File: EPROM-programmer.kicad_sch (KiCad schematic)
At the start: 34 parts, among them J1 ZIF-socket, J2 ISP, J3 DAC_A, J4 DAC_B, J5 GND, P1 USB-C, SW1 SW_Push, U1 ATmega1284-P, U2 MCP2221AxP, U3 MCP4812, Y1 20M

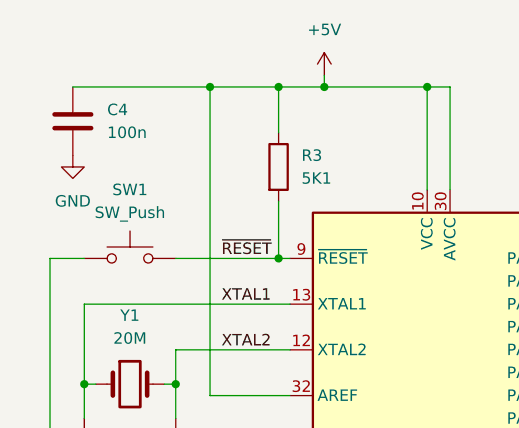
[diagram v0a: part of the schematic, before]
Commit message: Fix capacitor-stuff
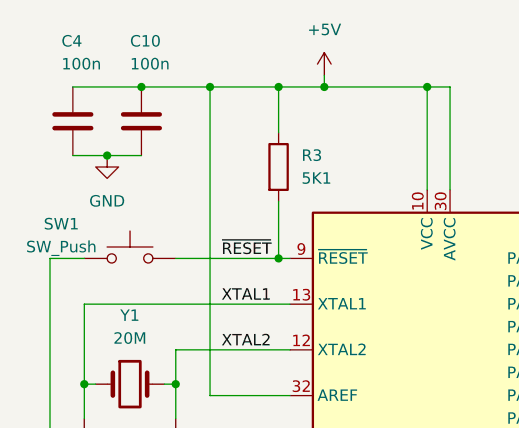
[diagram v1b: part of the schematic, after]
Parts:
- added C10: 100n, Capacitor_THT:C_Rect_L4.6mm_W3.0mm_P2.50mm_MKS02_FKP02, symbol Device:C
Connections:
- net +5V: now also C10.1
- net GND: now also C10.2
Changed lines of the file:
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@@
   (junction (at 99.06 157.48) (diameter 0) (color 0 0 0 0)
   )
+  (junction (at 25.4 35.56) (diameter 0) (color 0 0 0 0)
+  )
   (junction (at 180.34 154.94) (diameter 0) (color 0 0 0 0)
   )
@@
   )
   (junction (at 195.58 121.92) (diameter 0) (color 0 0 0 0)
+  )
+  (junction (at 21.59 43.18) (diameter 0) (color 0 0 0 0)
   )
   (junction (at 233.68 106.68) (diameter 0) (color 0 0 0 0)
@@
     (stroke (width 0) (type default))
   )
+  (wire (pts (xy 21.59 43.18) (xy 25.4 43.18))
+    (stroke (width 0) (type default))
+  )
   (wire (pts (xy 72.39 72.39) (xy 80.01 72.39))
     (stroke (width 0) (type default))
@@
     (stroke (width 0) (type default))
   )
-  (wire (pts (xy 17.78 35.56) (xy 33.02 35.56))
+  (wire (pts (xy 17.78 35.56) (xy 25.4 35.56))
     (stroke (width 0) (type default))
   )
@@
     (stroke (width 0) (type default))
   )
+  (wire (pts (xy 17.78 43.18) (xy 21.59 43.18))
+    (stroke (width 0) (type default))
+  )
   (wire (pts (xy 195.58 121.92) (xy 215.9 121.92))
     (stroke (width 0) (type default))
@@
     (stroke (width 0) (type default))
   )
+  (wire (pts (xy 25.4 35.56) (xy 33.02 35.56))
+    (stroke (width 0) (type default))
+  )
   (wire (pts (xy 132.08 176.53) (xy 143.51 176.53))
     (stroke (width 0) (type default))
@@
   )
   (symbol (lib_id "Device:C") (at 17.78 39.37 0) (unit 1)
-    (in_bom yes) (on_board yes) (dnp no) (fields_autoplaced)
-    (property "Reference" "C4" (at 21.59 38.1 0)
-      (effects (font (size 1.27 1.27)) (justify left))
-    )
-    (property "Value" "100n" (at 21.59 40.64 0)
+    (in_bom yes) (on_board yes) (dnp no)
+    (property "Reference" "C4" (at 16.51 30.48 0)
+      (effects (font (size 1.27 1.27)) (justify left))
+    )
+    (property "Value" "100n" (at 16.51 33.02 0)
       (effects (font (size 1.27 1.27)) (justify left))
     )
@@
     )
   )
-  (symbol (lib_id "power:GND") (at 17.78 43.18 0) (unit 1)
-    (in_bom yes) (on_board yes) (dnp no) (fields_autoplaced)
-    (property "Reference" "#PWR015" (at 17.78 49.53 0)
-      (effects (font (size 1.27 1.27)) hide)
-    )
-    (property "Value" "GND" (at 17.78 48.26 0)
-      (effects (font (size 1.27 1.27)))
-    )
-    (property "Footprint" "" (at 17.78 43.18 0)
-      (effects (font (size 1.27 1.27)) hide)
-    )
-    (property "Datasheet" "" (at 17.78 43.18 0)
+  (symbol (lib_id "power:GND") (at 21.59 43.18 0) (unit 1)
+    (in_bom yes) (on_board yes) (dnp no) (fields_autoplaced)
+    (property "Reference" "#PWR015" (at 21.59 49.53 0)
+      (effects (font (size 1.27 1.27)) hide)
+    )
+    (property "Value" "GND" (at 21.59 48.26 0)
+      (effects (font (size 1.27 1.27)))
+    )
+    (property "Footprint" "" (at 21.59 43.18 0)
+      (effects (font (size 1.27 1.27)) hide)
+    )
+    (property "Datasheet" "" (at 21.59 43.18 0)
       (effects (font (size 1.27 1.27)) hide)
     )
@@
   )
   (symbol (lib_id "Switch:SW_Push") (at 24.13 54.61 0) (unit 1)
-    (in_bom yes) (on_board yes) (dnp no) (fields_autoplaced)
-    (property "Reference" "SW1" (at 24.13 46.99 0)
-      (effects (font (size 1.27 1.27)))
-    )
-    (property "Value" "SW_Push" (at 24.13 49.53 0)
+    (in_bom yes) (on_board yes) (dnp no)
+    (property "Reference" "SW1" (at 16.51 50.8 0)
+      (effects (font (size 1.27 1.27)))
+    )
+    (property "Value" "SW_Push" (at 16.51 53.34 0)
       (effects (font (size 1.27 1.27)))
     )
@@
         )
       )
+    )
+  )
+  (symbol (lib_id "Device:C") (at 25.4 39.37 0) (unit 1)
+    (in_bom yes) (on_board yes) (dnp no)
+    (property "Reference" "C10" (at 24.13 30.48 0)
+      (effects (font (size 1.27 1.27)) (justify left))
+    )
+    (property "Value" "100n" (at 24.13 33.02 0)
+      (effects (font (size 1.27 1.27)) (justify left))
+    )
+    (property "Footprint" "Capacitor_THT:C_Rect_L4.6mm_W3.0mm_P2.50mm_MKS02_FKP02" (at 26.3652 43.18 0)
+      (effects (font (size 1.27 1.27)) hide)
+    )
+    (property "Datasheet" "~" (at 25.4 39.37 0)
+      (effects (font (size 1.27 1.27)) hide)
+    )
+    (pin "1")
+    (pin "2")
+    (instances
+      (project "EPROM-programmer"
+        (path "/8c5576b1-cb3e-4456-837b-2f47818a03ab"
+          (reference "C10") (unit 1)
+        )
+      )
